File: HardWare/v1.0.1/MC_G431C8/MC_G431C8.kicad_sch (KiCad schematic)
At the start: 19 parts, among them J2 Conn_01x03, J3 Conn_01x04, J4 Conn_01x06, U1 STM32G431C8, Y1 32MHZ

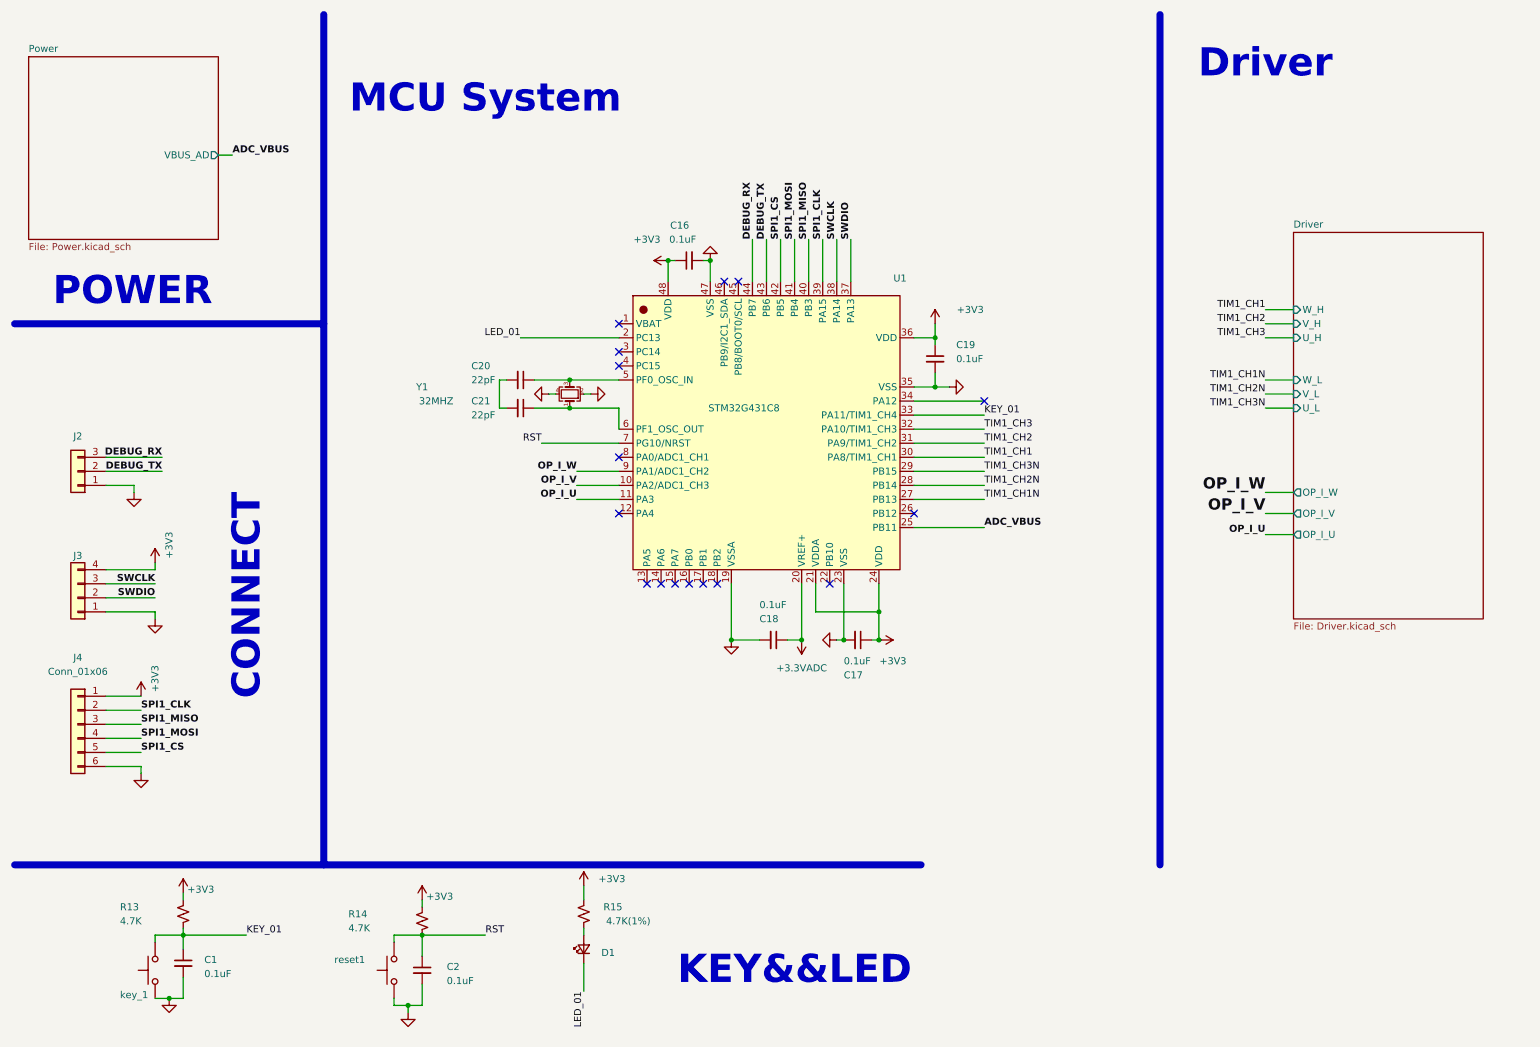
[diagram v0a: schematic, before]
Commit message: 20240604 优化硬件原理图及封装
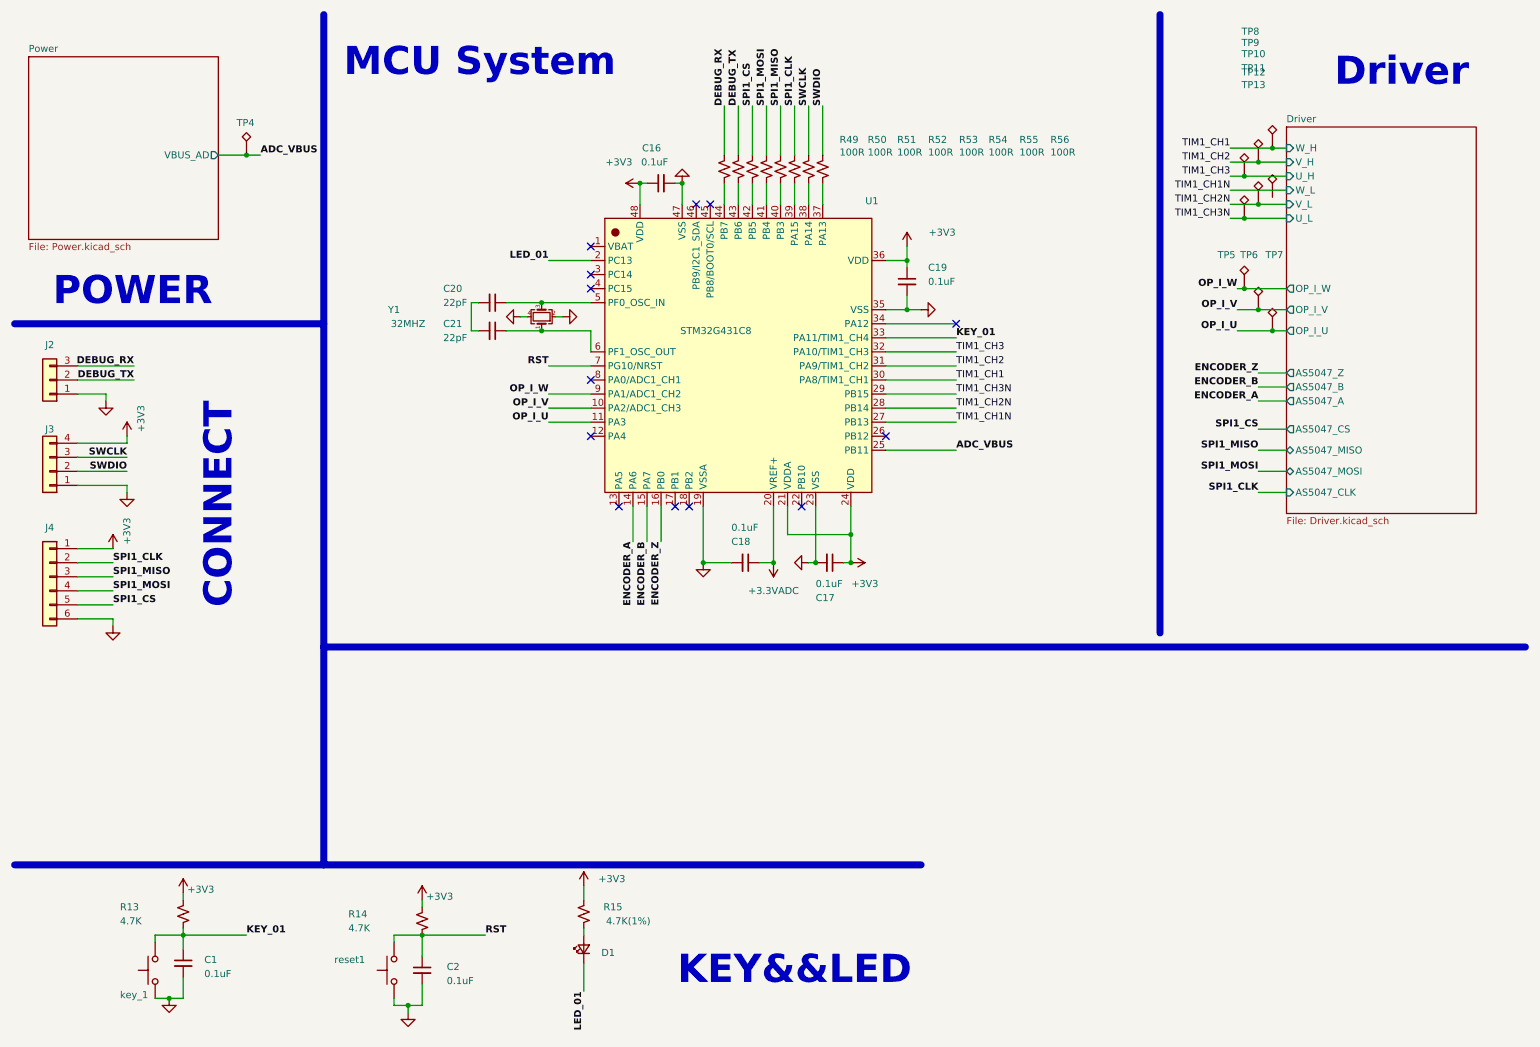
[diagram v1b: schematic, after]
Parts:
- added R49, R50, R51, R52, R53, R54, R55, R56: 100R, Resistor_SMD:R_0603_1608Metric, symbol Device:R_Small_US
- added TP10, TP11, TP12, TP13, TP4, TP5, TP6, TP7, TP8, TP9: TestPoint_Alt, TestPoint:TestPoint_Pad_D1.0mm, symbol Connector:TestPoint_Alt
- J2: footprint Connector_PinHeader_2.54mm:PinHeader_1x03_P2.54mm_Vertical -> Connector_Molex:Molex_PicoBlade_53398-0371_1x03-1MP_P1.25mm_Vertical
- J3: footprint Connector_PinHeader_2.54mm:PinHeader_1x04_P2.54mm_Vertical -> Connector_Molex:Molex_PicoBlade_53398-0471_1x04-1MP_P1.25mm_Vertical
- J4: footprint Connector_PinHeader_2.54mm:PinHeader_1x06_P2.54mm_Vertical -> Connector_Molex:Molex_PicoBlade_53398-0671_1x06-1MP_P1.25mm_Vertical
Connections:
- net ADC_VBUS: now also TP4.1
- net DEBUG_RX: now also R49.1; no longer U1.44 (PB7)
- net DEBUG_TX: now also R50.1; no longer U1.43 (PB6)
- net OP_I_U: now also TP7.1
- net OP_I_V: now also TP6.1
- net OP_I_W: now also TP5.1
- net SPI1_CLK: now also R54.1; no longer U1.39 (PA15)
- net SPI1_CS: now also R51.1; no longer U1.42 (PB5)
- net SPI1_MISO: now also R53.1; no longer U1.40 (PB3)
- net SPI1_MOSI: now also R52.1; no longer U1.41 (PB4)
- net SWCLK: now also R55.1; no longer U1.38 (PA14)
- net SWDIO: now also R56.1; no longer U1.37 (PA13)
- net TIM1_CH1: now also TP8.1
- net TIM1_CH2: now also TP9.1
- net TIM1_CH2N: now also TP12.1
- net TIM1_CH3: now also TP10.1
- net TIM1_CH3N: now also TP13.1
- net ENCODER_A: now reaches U1.14 (PA6)
- net ENCODER_B: now reaches U1.15 (PA7)
- net ENCODER_Z: now reaches U1.16 (PB0)
- new net: R56.2, U1.37 (PA13)
- new net: R55.2, U1.38 (PA14)
- new net: R54.2, U1.39 (PA15)
- new net: R53.2, U1.40 (PB3)
- new net: R52.2, U1.41 (PB4)
- new net: R51.2, U1.42 (PB5)
- new net: R50.2, U1.43 (PB6)
- new net: R49.2, U1.44 (PB7)
- no-connect marks 16 -> 13
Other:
- sheet Driver ports: added AS5047_A, AS5047_B, AS5047_CLK, AS5047_CS, AS5047_MISO, AS5047_MOSI, AS5047_Z; removed none
- moved on the sheet: C16, C17, C18, C19, C20, C21, J2, J3, J4, U1, Y1
